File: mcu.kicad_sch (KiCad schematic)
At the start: 48 parts, among them SW1 SW_Push, SW2 SW_Push, U2 ESP32-S3-WROOM-1, U3 SN74AXC4T245PWR, U4 TCA9517DGKR, Y1 32.768kHz

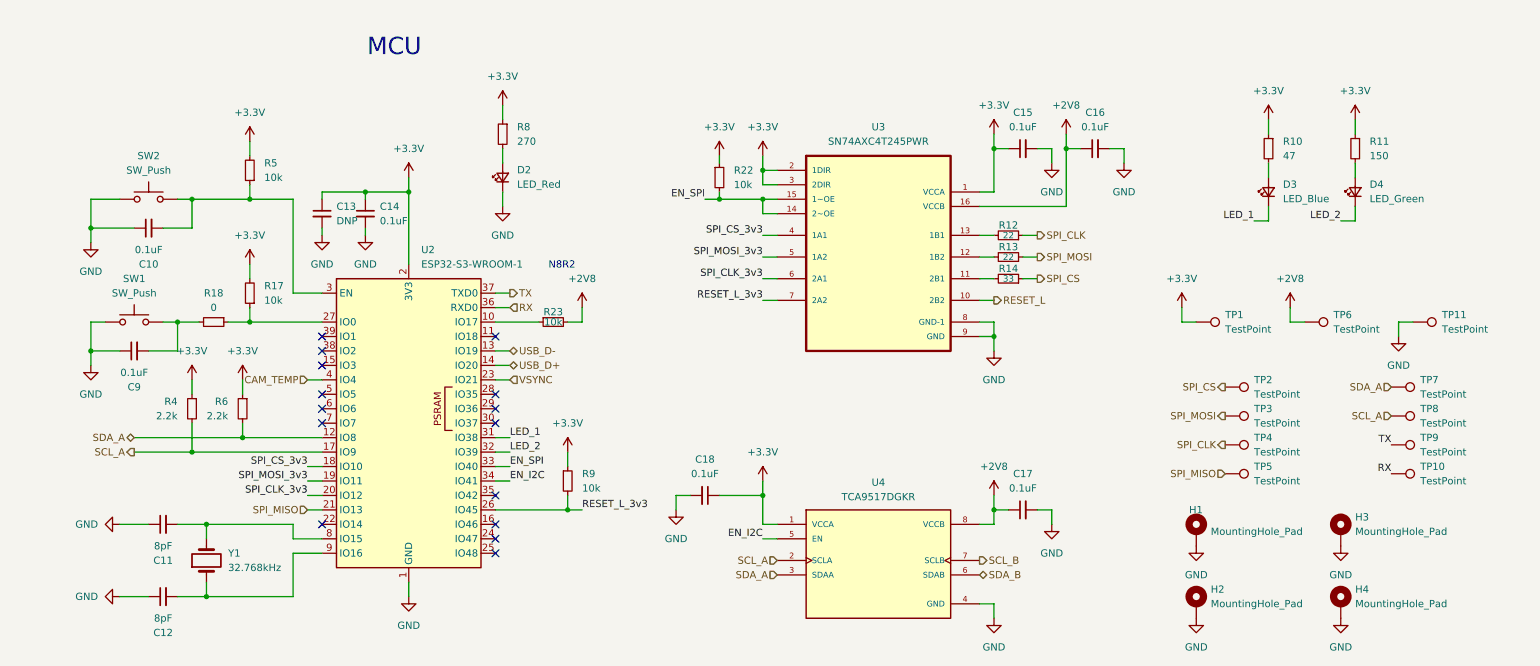
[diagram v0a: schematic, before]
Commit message: Rev A PCB Ordered
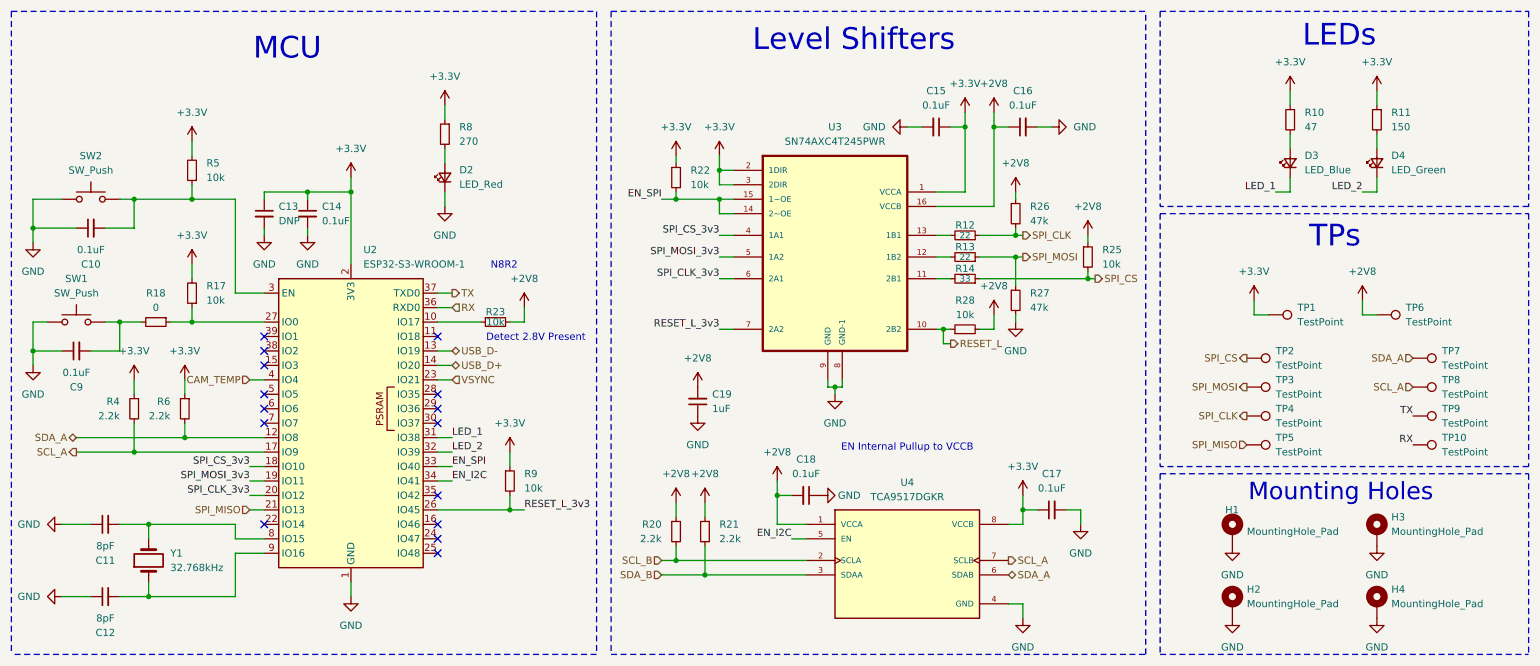
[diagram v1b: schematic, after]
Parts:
- removed TP11: TestPoint, TestPoint:TestPoint_THTPad_1.5x1.5mm_Drill0.7mm, symbol Connector:TestPoint
- added C19: 1uF, Capacitor_SMD:C_0805_2012Metric_Pad1.18x1.45mm_HandSolder, symbol Device:C_Small
- added R20, R21: 2.2k, Resistor_SMD:R_0805_2012Metric_Pad1.20x1.40mm_HandSolder, symbol Device:R_Small
- added R25, R28: 10k, Resistor_SMD:R_0805_2012Metric_Pad1.20x1.40mm_HandSolder, symbol Device:R_Small
- added R26, R27: 47k, Resistor_SMD:R_0805_2012Metric_Pad1.20x1.40mm_HandSolder, symbol Device:R_Small
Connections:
- net +2V8: now also C18.2, U4.1 (VCCA), C19.2, R20.1, R21.1, R25.1, R26.1, R28.2; no longer C17.1, U4.8 (VCCB)
- net +3.3V: now also C17.1, U4.8 (VCCB); no longer C18.1, U4.1 (VCCA)
- net GND: now also C18.1, C19.1, R27.2; no longer C18.2
- net RESET_L: now also R28.1
- net SCL_A: now also U4.7 (SCLB); no longer U4.2 (SCLA)
- net SCL_B: now also U4.2 (SCLA), R20.2; no longer U4.7 (SCLB)
- net SDA_A: now also U4.6 (SDAB); no longer U4.3 (SDAA)
- net SDA_B: now also U4.3 (SDAA), R21.2; no longer U4.6 (SDAB)
- net SPI_CLK: now also R26.2
- net SPI_CS: now also R25.2
- net SPI_MOSI: now also R27.1
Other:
- note added: "Detect 2.8V Present"
- note added: "EN Internal Pullup to VCCB"
- note added: "LEDs"
- note added: "Level Shifters"
- note added: "Mounting Holes"
- note added: "TPs"
- company: (none) -> FrostByte Solutions
- title: (none) -> FrostByte IR Camera Interface Board
- moved on the sheet: C10, C11, C12, C13, C14, C15, C16, C17, C18, C9, D2, D3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
